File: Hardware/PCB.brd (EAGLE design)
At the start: 46 x 35 mm, 105 parts, among them IC1 BQ25180YBGR, IC2 DRV2605YZFR, IC3 BMA421, IC9 RT6160AWSC, J1 503480-2400, J2 TC2030-IDC, J4 KH-TYPE-C-16P, Q3 SI1308EDL-T1-GE3, U1 NRF52840_QF, U3 MAX17048G+T10, X1 32MHz, X2 32.768kHz

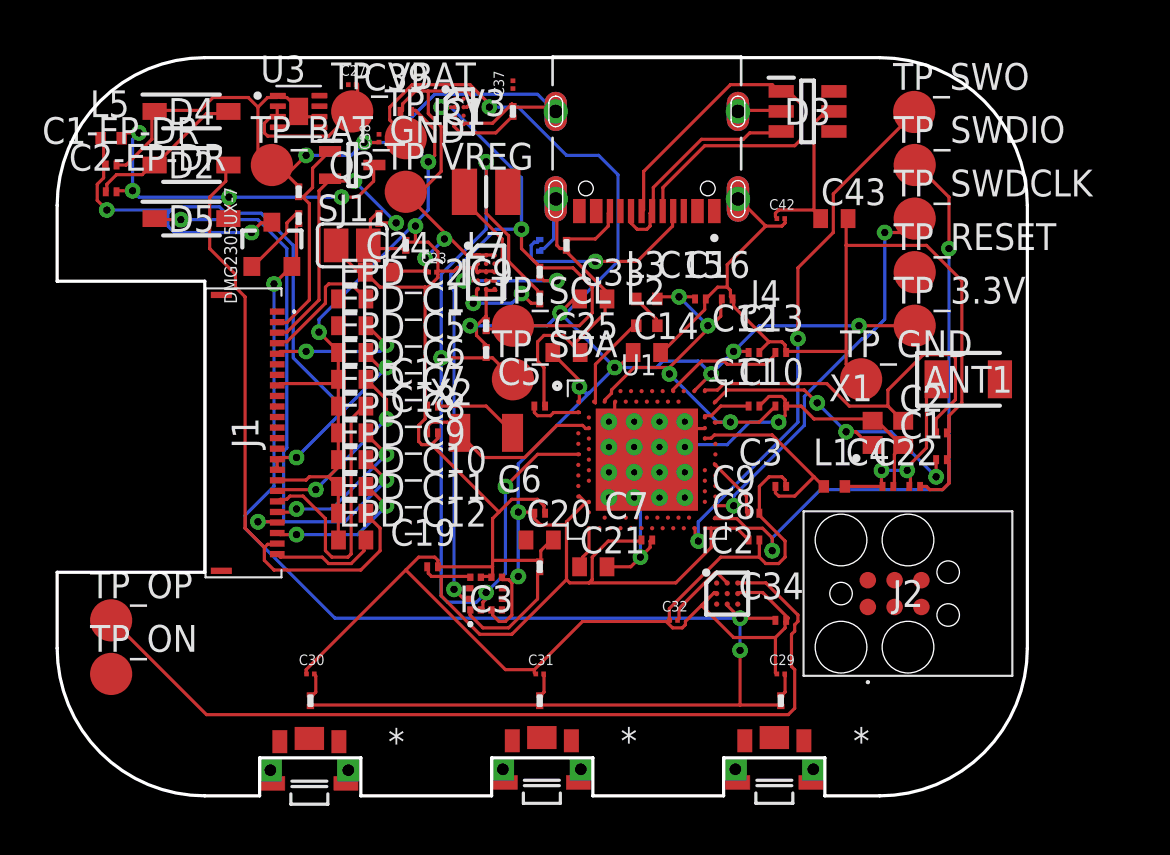
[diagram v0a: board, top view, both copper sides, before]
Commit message: Fixed 4 issues
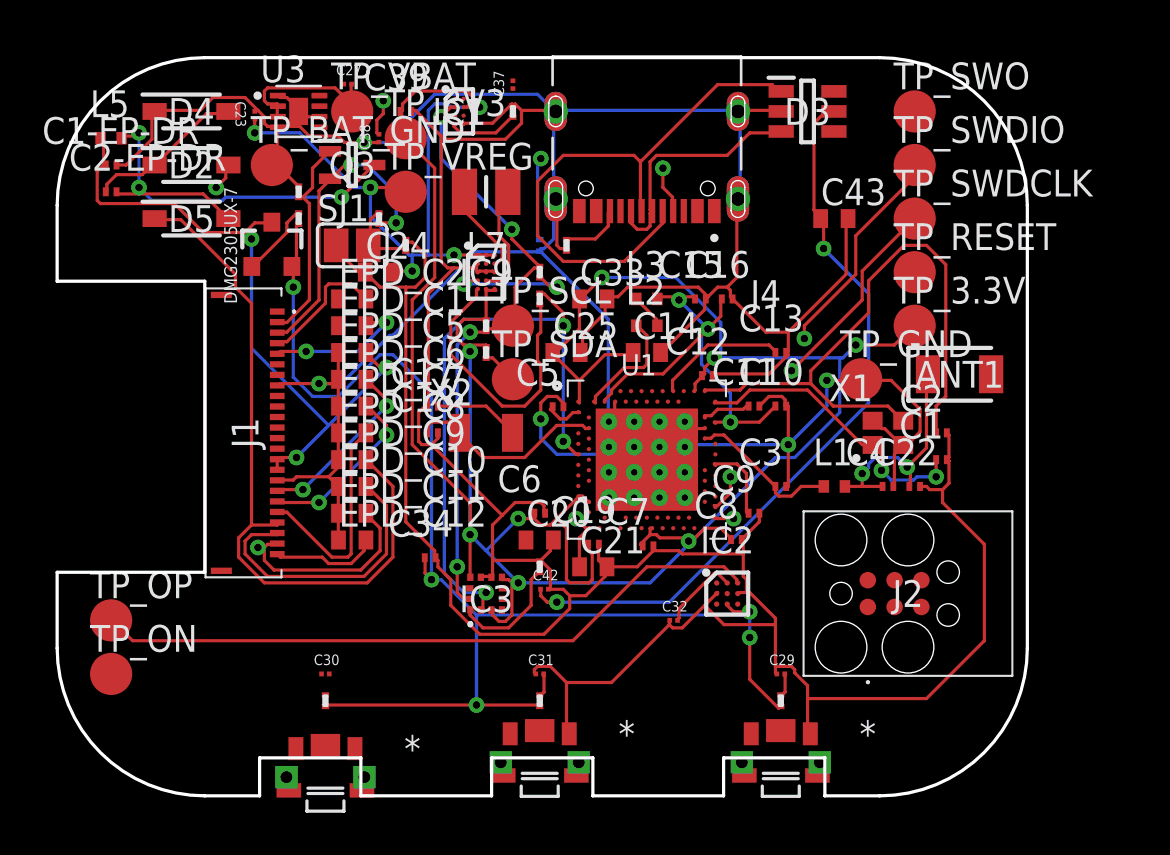
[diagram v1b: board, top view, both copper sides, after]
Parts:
- moved C42 20.8 mm to (52.3, 117.0)
- moved C34 16.9 mm to (46.9, 118.5)
- moved C23 11.2 mm to (38.6, 139.5), turned to 90.7 degrees
- moved C19 7.71 mm to (54.6, 119.2)
- moved C12 2.47 mm to (60.0, 127.2)
- moved C5 0.87 mm to (52.9, 125.7)
- moved C8 0.84 mm to (61.4, 119.4)
- moved SW_UP 0.83 mm to (41.9, 108.5)
- moved C30 0.71 mm to (41.9, 113.0)
- moved R5 0.71 mm to (41.9, 111.8)
- moved ANT1 0.48 mm to (72.0, 127.2)
- moved SW_DN 0.45 mm to (63.5, 109.2)
- moved SW_ENT 0.35 mm to (52.1, 109.2)
- moved C7 0.28 mm to (57.2, 119.1)
- moved C27 0.21 mm to (43.0, 141.0)
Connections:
- net VBUS/2.6D: now also IC1.A2
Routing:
- net GND: track 257.7 -> 332.0 mm, vias 7 -> 5
- net VBUS/1.5D: track 8.54 -> 35.5 mm, vias 0 -> 2
- net VBUS/2.6D: track 2.10 -> 28.2 mm, vias 0 -> 2
- net SWO: track 25.3 -> 0.00 mm, vias 2 -> 0
- net SDA/2.4C: track 45.7 -> 31.0 mm, vias 4 -> 3
- net VREG: track 20.8 -> 33.6 mm, vias 2 -> 5
- net SCL/2.4C: track 40.2 -> 29.0 mm, vias 3 -> 4
- net OUT+: track 42.5 -> 32.0 mm
- net N$15: track 19.0 -> 29.2 mm
- net N$3: track 4.31 -> 13.4 mm, vias 2 -> 0
- net SWDIO: track 29.7 -> 21.3 mm
- net 3V3/2.4A: track 107.5 -> 115.7 mm, vias 10 -> 8
- net 3V3/1.7D: track 69.9 -> 62.7 mm, vias 3 -> 5
- net N$32: track 7.12 -> 13.6 mm, vias 2 -> 0
- net EPD_3V3: track 37.2 -> 31.9 mm, vias 4 -> 3
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- added copper zone on layer 2, net VLAD
- removed copper zone on layer 2, net GND
